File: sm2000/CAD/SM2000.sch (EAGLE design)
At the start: 441 parts, among them CN1 HDR100-3, CN2 ST-3509, CN3 HDR100-3, CN4 JS-MU3-002, CN5 DS-0518, CN6 ST-3509, CN7 ST-3509, J1 JMP-2PIN, J10 JMPR-2X2, J11 JMPR-2X2, J12 JMPR-2X2, J13 JMPR-2X2, J14 JMPR-2X2, J2 HDR100-7, J3 JMP-2PIN, J4 CONN-BOOM-XH-2A, J5 JMP-2PIN, J6 JMPR-2X2, J7 JMPR-2X2, J8 JMPR-2X2, J9 JMPR-2X2, P6 TPAD50, P7 TPAD50, P8 TPAD50, P9 TPAD50, Q1 MMBT3904, Q10 MMBT3904, Q11 BFR92, Q12 BFQ19, Q13 RD01MUS2, Q14 MMBT3904, Q15 MMBT3904, Q16 MMBT3904, Q17 MMBT3906, Q2 STR2P3LLH6, Q3 MMBT3904, Q4 STR2P3LLH6, Q5 MMBT3904, Q6 MMBT3904, Q7 MMBT3904, Q8 MMBT3904, Q9 MMBT3904, SW1 TS-02B, SW2 SW-LC2259, SW3 TS-026, SW4 TS-026, SW5 SW-LC2259EENP, U1 STM32F405VGT6, U10 LM386M-1, U11 ADE-1, U12 PGA-103+, U13 LMV341, U14 SI5351A, U15 SI570, U16 SA612A, U2 STMPS2141, U3 EMIF02-USB03F2, U4 DNL, U5 L78M09, U6 LD1117AS-33, U7 LMV341, U8 LD1117AS-33, U9 TPS54329E, X1 BU-SMA-H

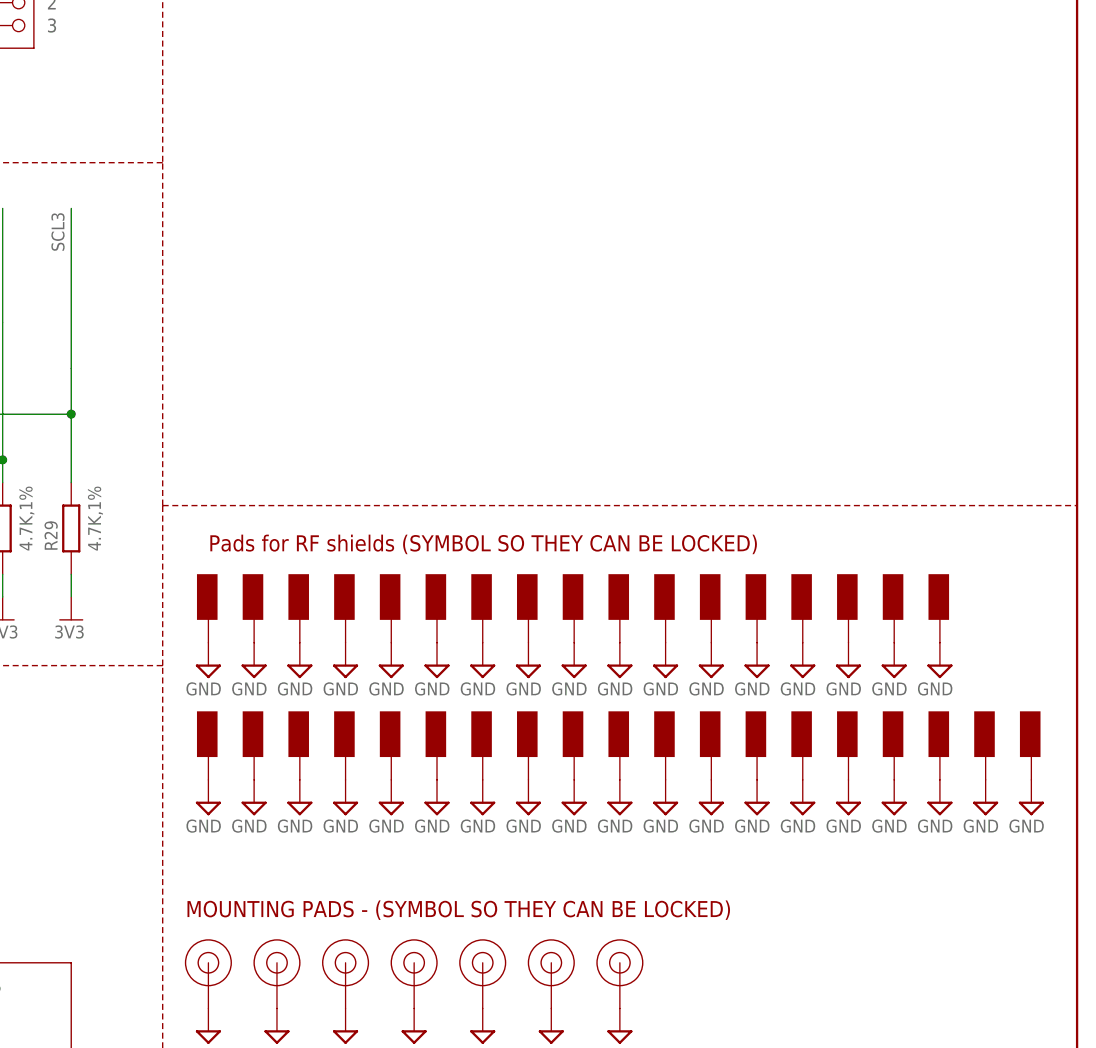
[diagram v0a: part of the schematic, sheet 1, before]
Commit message: LAYOUT UPDATES as of 4/13/16  RGB 80 NODES to COMPLETE
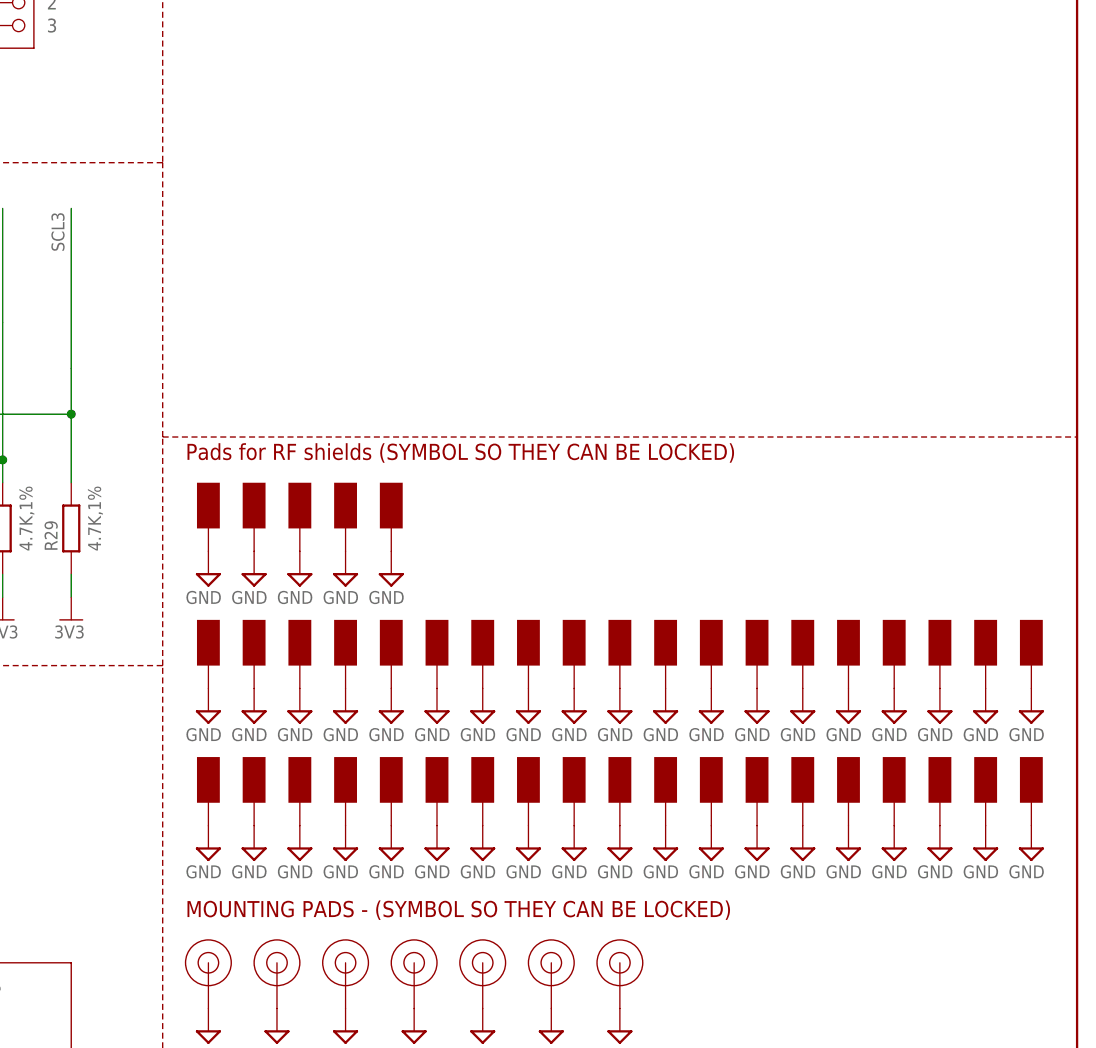
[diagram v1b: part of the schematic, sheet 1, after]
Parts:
- added S37, S38, S39, S40, S41, S42, S43: SGND, _RoweTel:SGND
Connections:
- net GND: now also S37.1, S38.1, S39.1, S40.1, S41.1, S42.1, S43.1
